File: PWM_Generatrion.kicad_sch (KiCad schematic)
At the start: 2 parts, among them J25 IPT1-105-01-L-D, U22 PCA9685PW_118

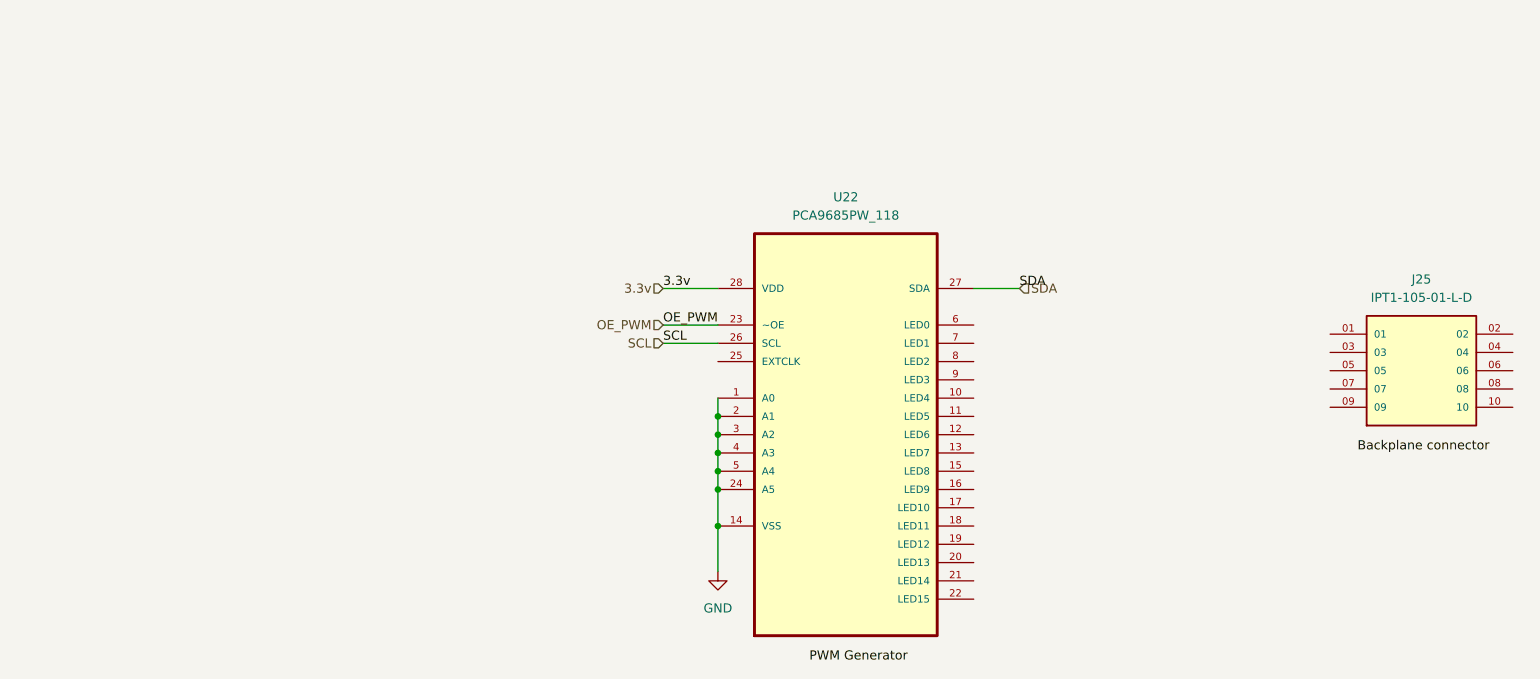
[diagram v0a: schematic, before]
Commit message: stuff
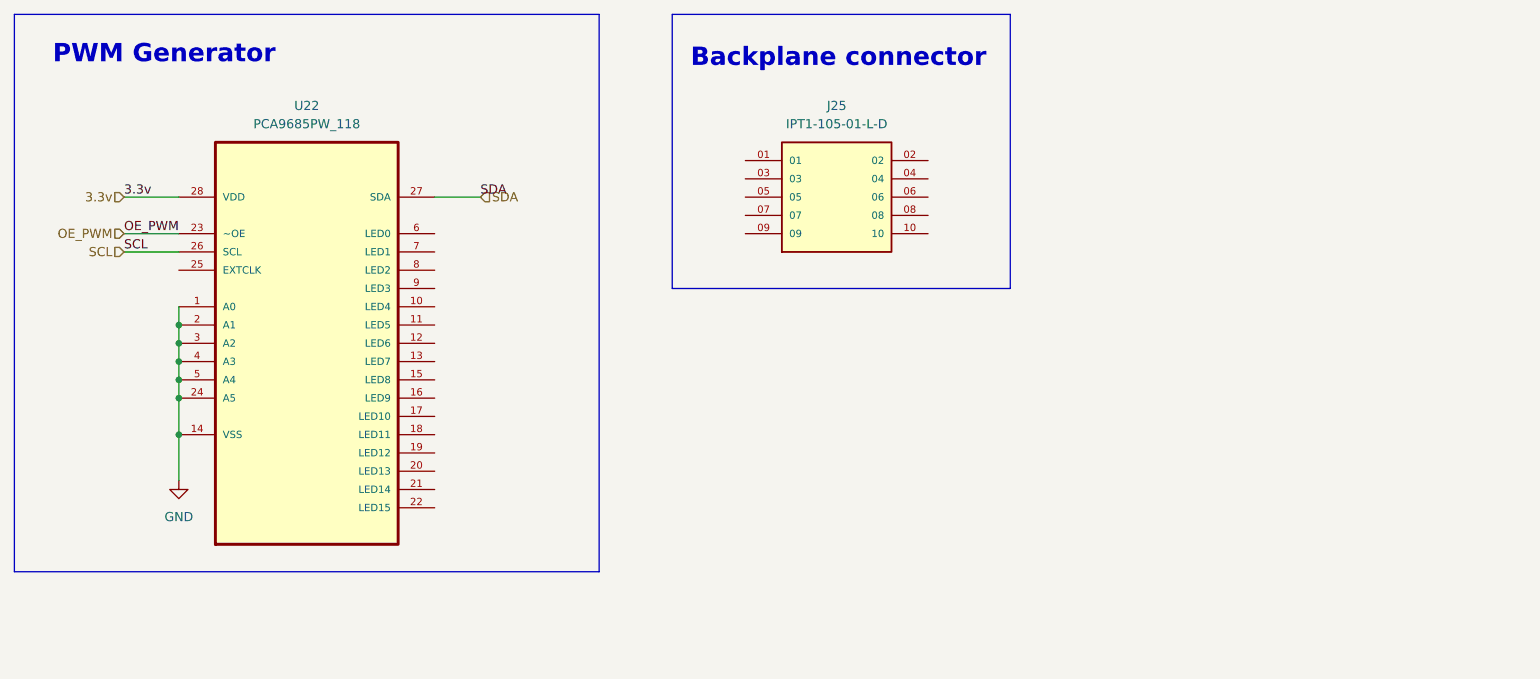
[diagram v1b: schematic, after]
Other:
- note added: "Backplane connector"
- note added: "PWM Generator"
- moved on the sheet: J25, U22
